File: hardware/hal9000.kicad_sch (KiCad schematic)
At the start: 13 parts

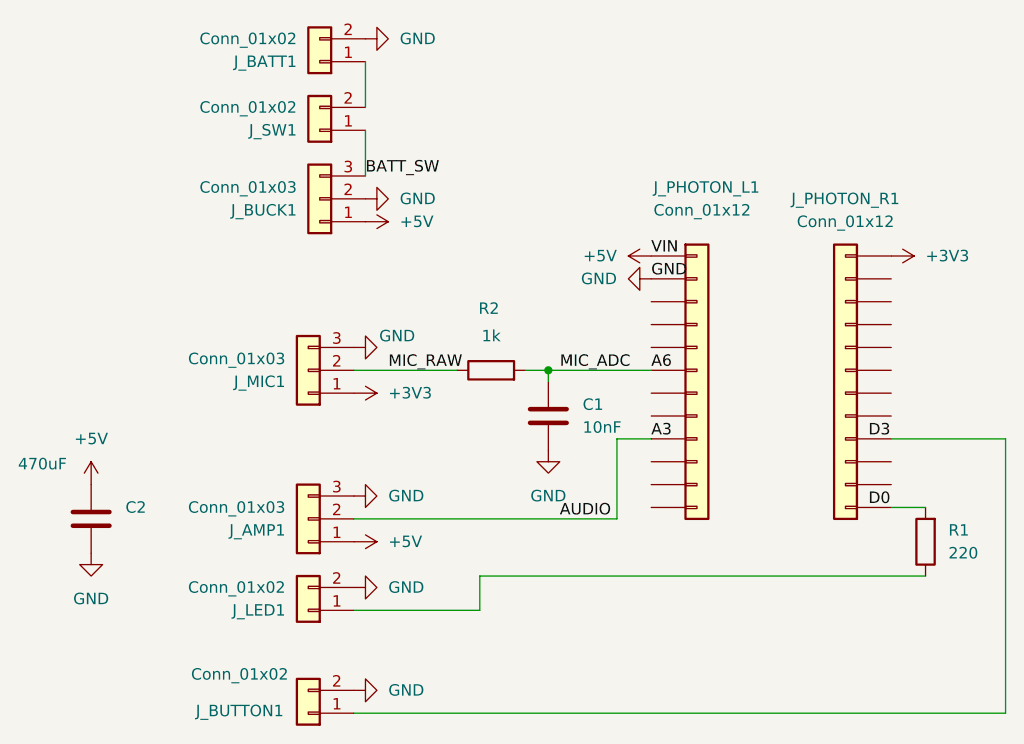
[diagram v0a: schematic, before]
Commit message: hw: reva2 kicad files
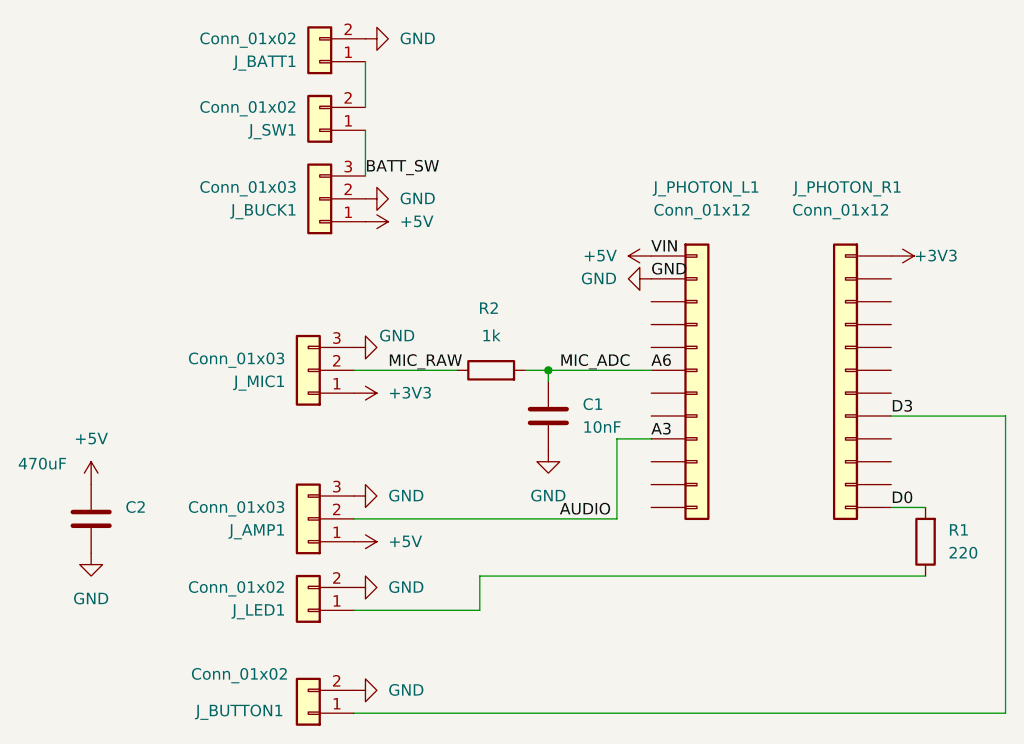
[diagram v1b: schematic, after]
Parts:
- C2: footprint Capacitor_SMD:C_0805_2012Metric_Pad1.18x1.45mm_HandSolder -> Capacitor_THT:CP_Radial_D6.3mm_P2.50mm
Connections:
- net +3V3: now also J_PHOTON_R1.1 (Pin_1); no longer J_PHOTON_R1.12 (Pin_12)
- net D0: now also J_PHOTON_R1.12 (Pin_12), R1.2
- net D3: now also J_BUTTON1.1 (Pin_1), J_PHOTON_R1.8 (Pin_8)
- net at J_PHOTON_R1.4 (Pin_4): no longer J_BUTTON1.1 (Pin_1)
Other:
- moved on the sheet: J_PHOTON_R1
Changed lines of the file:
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@@
 	(wire
 		(pts
-			(xy 180.34 121.92) (xy 167.64 121.92)
+			(xy 180.34 119.38) (xy 167.64 119.38)
 		)
 		(stroke
@@
 	(wire
 		(pts
-			(xy 107.95 140.97) (xy 121.92 140.97)
+			(xy 167.64 129.54) (xy 171.45 129.54)
 		)
 		(stroke
@@
 	(wire
 		(pts
-			(xy 109.22 80.01) (xy 109.22 85.09)
+			(xy 107.95 140.97) (xy 121.92 140.97)
 		)
 		(stroke
@@
 	(wire
 		(pts
-			(xy 129.54 114.3) (xy 140.97 114.3)
+			(xy 109.22 80.01) (xy 109.22 85.09)
 		)
 		(stroke
@@
 	(wire
 		(pts
-			(xy 167.64 129.54) (xy 171.45 129.54)
+			(xy 129.54 114.3) (xy 140.97 114.3)
 		)
 		(stroke
@@
 	(wire
 		(pts
-			(xy 180.34 152.4) (xy 180.34 121.92)
+			(xy 180.34 152.4) (xy 180.34 119.38)
 		)
 		(stroke
@@
 	)
 	(label "D0"
-		(at 165.1 129.54 0)
+		(at 167.64 129.54 0)
 		(effects
 			(font
@@
 	)
 	(label "D3"
-		(at 165.1 121.92 0)
+		(at 167.64 119.38 0)
 		(effects
 			(font
@@
 		)
 		(property "Value" "+3V3"
-			(at 171.45 101.5999 90)
+			(at 170.18 101.6 90)
 			(effects
 				(font
@@
 			)
 		)
-		(property "Footprint" "Capacitor_SMD:C_0805_2012Metric_Pad1.18x1.45mm_HandSolder"
+		(property "Footprint" "Capacitor_THT:CP_Radial_D6.3mm_P2.50mm"
 			(at 79.7052 134.62 0)
 			(effects
@@
 			)
 		)
-		(property "Description" "Unpolarized capacitor"
+		(property "Description" ""
 			(at 78.74 130.81 0)
 			(effects
@@
 	(symbol
 		(lib_id "Connector_Generic:Conn_01x12")
-		(at 162.56 116.84 180)
-		(unit 1)
-		(exclude_from_sim no)
-		(in_bom yes)
-		(on_board yes)
-		(dnp no)
-		(fields_autoplaced yes)
+		(at 162.56 114.3 0)
+		(mirror y)
+		(unit 1)
+		(exclude_from_sim no)
+		(in_bom yes)
+		(on_board yes)
+		(dnp no)
 		(property "Reference" "J_PHOTON_R1"
-			(at 162.56 95.25 0)
+			(at 162.814 93.98 0)
 			(effects
 				(font
@@
 		)
 		(property "Value" "Conn_01x12"
-			(at 162.56 97.79 0)
+			(at 162.052 96.52 0)
 			(effects
 				(font
@@
 		)
 		(property "Footprint" "Connector_PinSocket_2.54mm:PinSocket_1x12_P2.54mm_Vertical"
-			(at 162.56 116.84 0)
+			(at 162.56 114.3 0)
 			(effects
 				(font
@@
 		)
 		(property "Datasheet" "~"
-			(at 162.56 116.84 0)
+			(at 162.56 114.3 0)
 			(effects
 				(font
@@
 		)
 		(property "Description" "Generic connector, single row, 01x12, script generated (kicad-library-utils/schlib/autogen/connector/)"
-			(at 162.56 116.84 0)
-			(effects
-				(font
+			(at 162.56 114.3 0)
+			(effects
+				(font
